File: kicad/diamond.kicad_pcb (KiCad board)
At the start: 2 copper layers, 76.5 x 66.3 mm, 40 parts, among them J1 INPUT, Q1 BD139, Q2 BD140, Q3 NJW0281G, Q4 NJW0302G, U1 NE5532

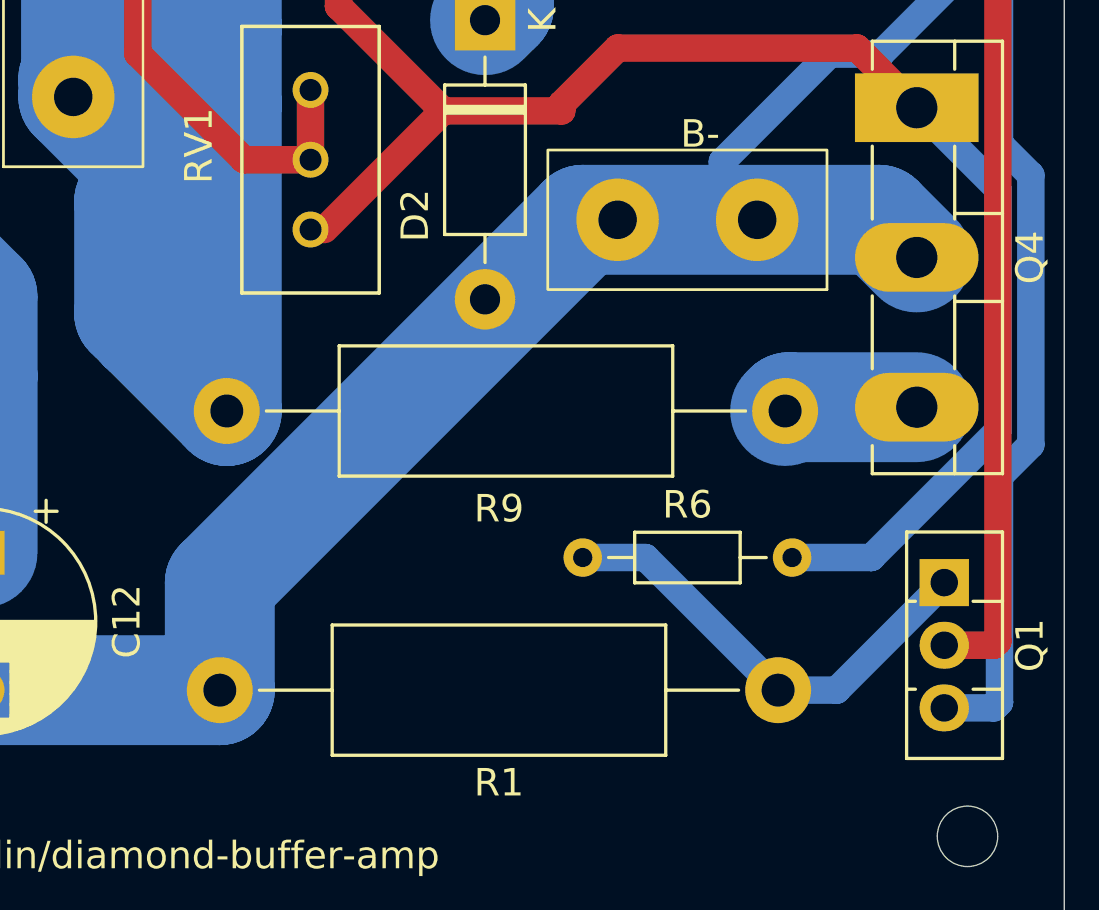
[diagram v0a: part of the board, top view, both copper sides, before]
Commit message: WIP
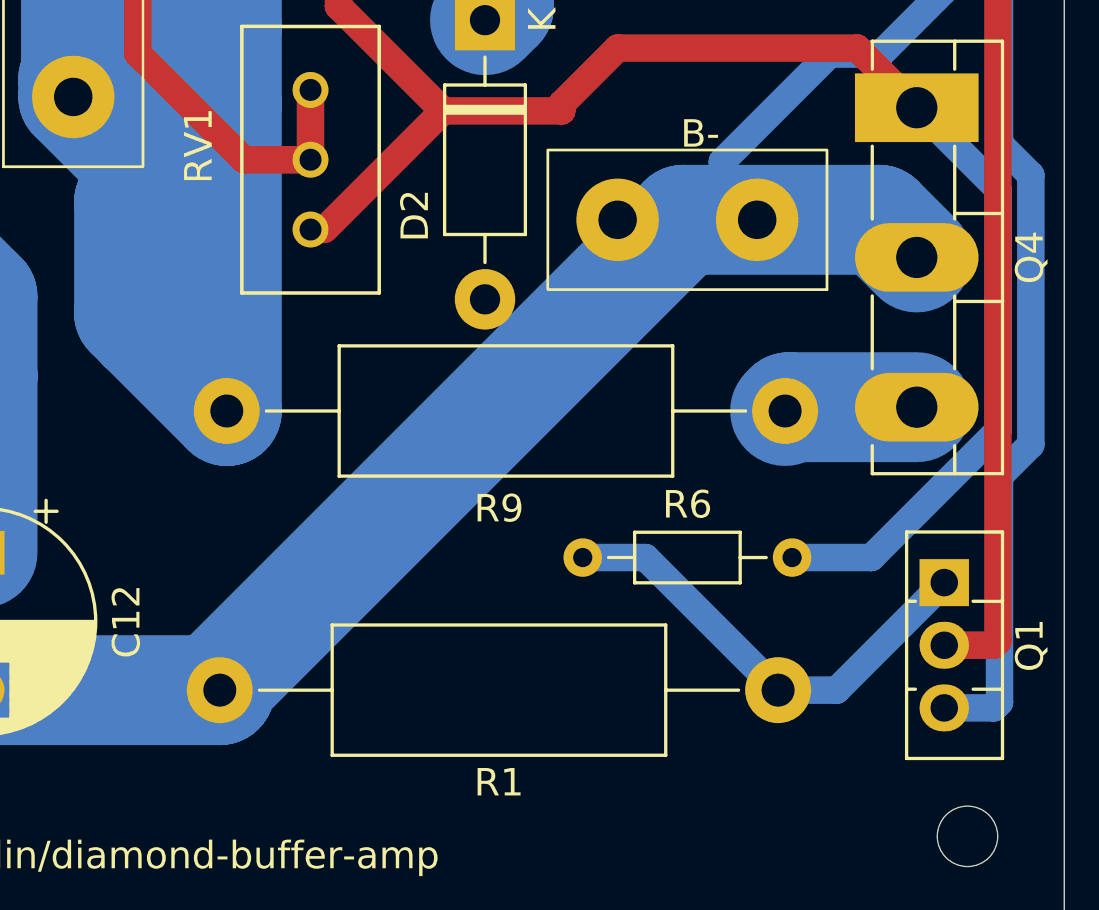
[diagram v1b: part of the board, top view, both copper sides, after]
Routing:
- net B-: track 126.9 -> 124.7 mm
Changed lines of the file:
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@@
 			(outputformat 1)
 			(mirror no)
-			(drillshape 1)
+			(drillshape 0)
 			(scaleselection 1)
-			(outputdirectory "")
+			(outputdirectory "gerber")
 		)
 	)
@@
 	)
 	(segment
-		(start 145.288 102.77)
-		(end 158.496 89.562)
-		(width 4)
+		(start 171.654 58.298)
+		(end 170.053 59.899)
+		(width 1)
 		(layer "B.Cu")
 		(net 18)
 	)
 	(segment
-		(start 171.654 58.298)
-		(end 170.053 59.899)
-		(width 1)
+		(start 145.288 106.68)
+		(end 145.288 106.426)
+		(width 4)
 		(layer "B.Cu")
 		(net 18)
@@
 	)
 	(segment
+		(start 145.288 106.426)
+		(end 162.152 89.562)
+		(width 4)
+		(layer "B.Cu")
+		(net 18)
+	)
+	(segment
+		(start 169.284 89.562)
+		(end 170.654 90.932)
+		(width 4)
+		(layer "B.Cu")
+		(net 18)
+	)
+	(segment
 		(start 169.337791 83.531)
 		(end 167.48568 83.531)
@@
 	)
 	(segment
-		(start 145.288 106.68)
-		(end 145.288 102.77)
+		(start 162.152 89.562)
+		(end 169.284 89.562)
 		(width 4)
 		(layer "B.Cu")
@@
 	)
 	(segment
-		(start 169.284 89.562)
-		(end 170.654 90.932)
-		(width 4)
-		(layer "B.Cu")
-		(net 18)
-	)
-	(segment
 		(start 170.053 59.899)
 		(end 170.053 61.575)
@@
 		(layer "B.Cu")
 		(net 18)
-	)
-	(segment
-		(start 158.496 89.562)
-		(end 169.284 89.562)
-		(width 4)
-		(layer "B.Cu")
-		(net 18)

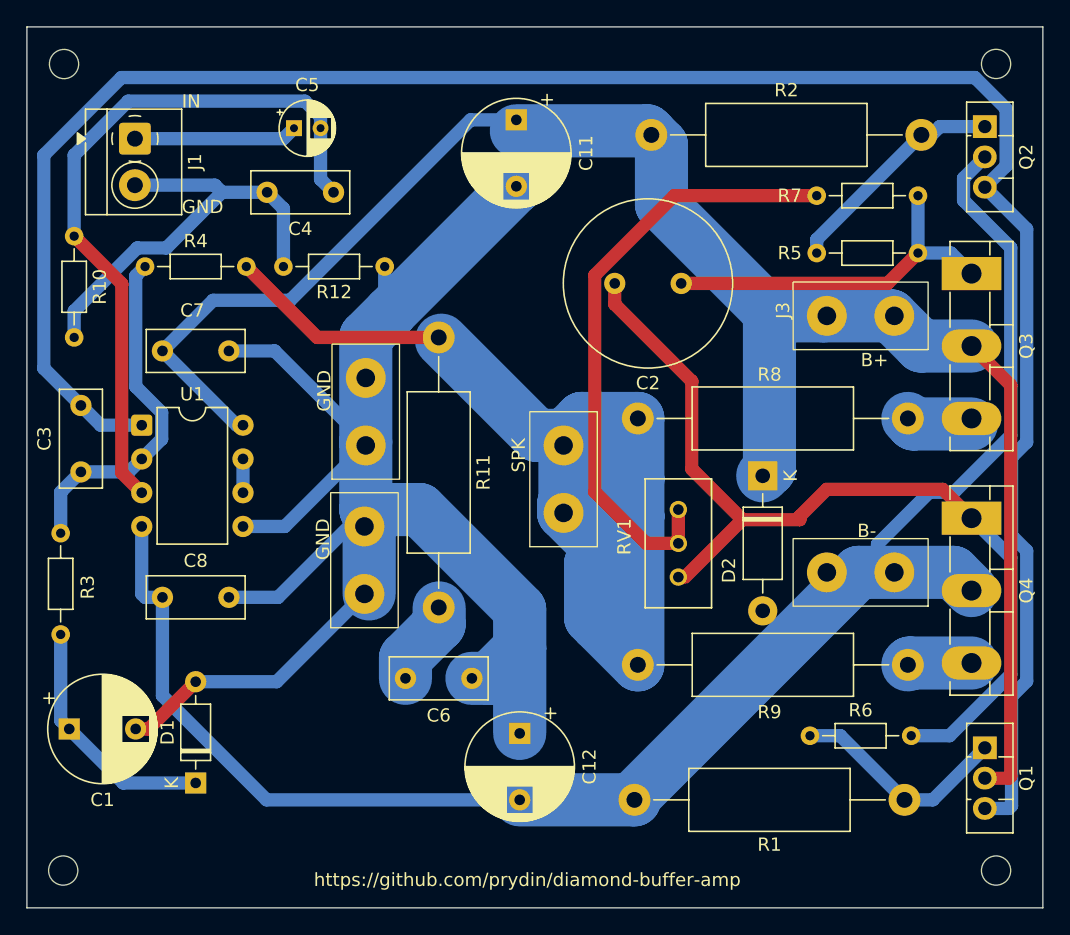
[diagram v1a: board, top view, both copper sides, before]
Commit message: WIP
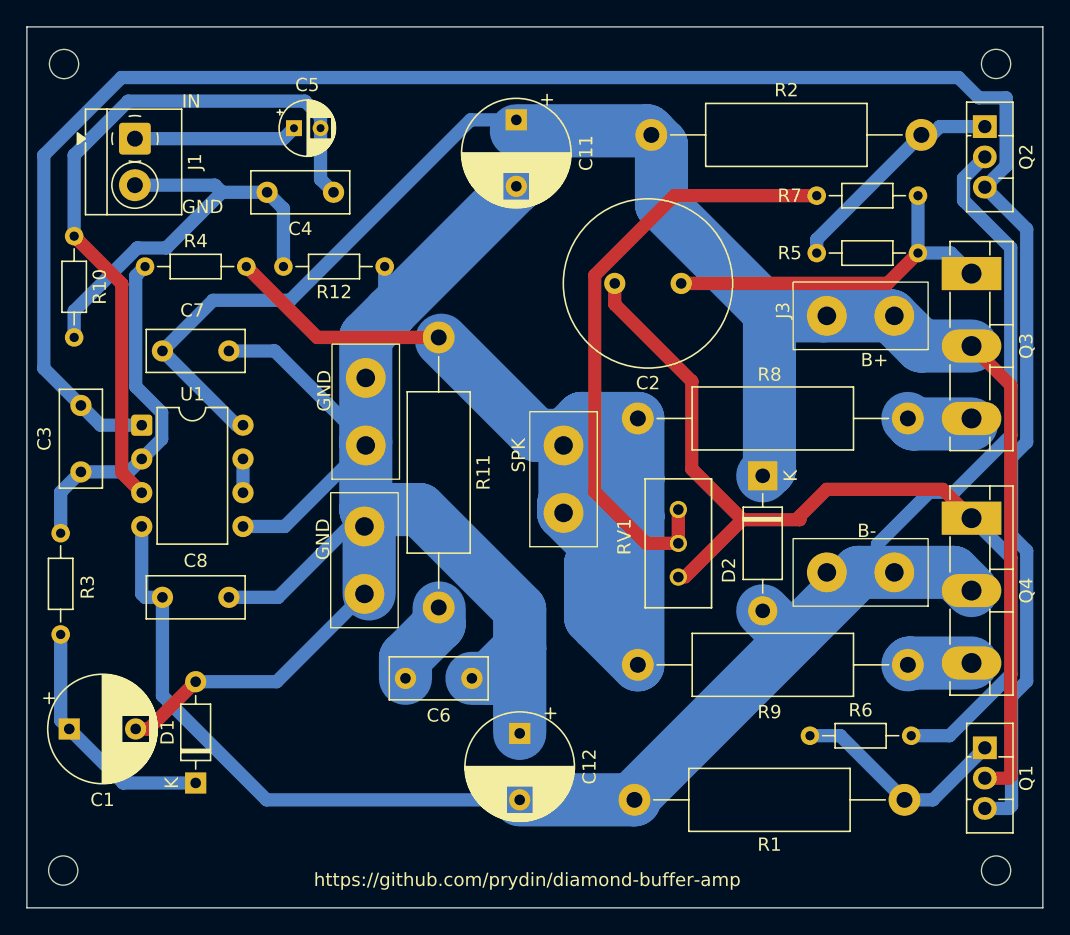
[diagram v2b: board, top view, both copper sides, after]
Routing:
- net B-: track 124.7 -> 128.0 mm
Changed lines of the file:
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@@
 	)
 	(segment
-		(start 173.255 54.672709)
-		(end 173.255 58.977)
+		(start 169.672 52.324)
+		(end 171.196 53.848)
+		(width 1)
+		(layer "B.Cu")
+		(net 3)
+	)
+	(segment
+		(start 100.838 58.166)
+		(end 106.68 52.324)
+		(width 1)
+		(layer "B.Cu")
+		(net 3)
+	)
+	(segment
+		(start 106.68 52.324)
+		(end 169.672 52.324)
 		(width 1)
 		(layer "B.Cu")
@@
 	)
 	(segment
+		(start 173.255 53.848)
+		(end 173.255 58.977)
+		(width 1)
+		(layer "B.Cu")
+		(net 3)
+	)
+	(segment
+		(start 171.196 53.848)
+		(end 173.255 53.848)
+		(width 1)
+		(layer "B.Cu")
+		(net 3)
+	)
+	(segment
+		(start 174.805 79.760847)
+		(end 174.805 63.729)
+		(width 1)
+		(layer "B.Cu")
+		(net 3)
+	)
+	(segment
+		(start 171.654 107.326)
+		(end 173.464 107.326)
+		(width 1)
+		(layer "B.Cu")
+		(net 3)
+	)
+	(segment
+		(start 173.666 86.796944)
+		(end 173.666 80.899847)
+		(width 1)
+		(layer "B.Cu")
+		(net 3)
+	)
+	(segment
+		(start 108.209 78.486)
+		(end 105.116 78.486)
+		(width 1)
+		(layer "B.Cu")
+		(net 3)
+	)
+	(segment
+		(start 103.632 77.002)
+		(end 100.838 74.208)
+		(width 1)
+		(layer "B.Cu")
+		(net 3)
+	)
+	(segment
+		(start 105.116 78.486)
+		(end 103.632 77.002)
+		(width 1)
+		(layer "B.Cu")
+		(net 3)
+	)
+	(segment
+		(start 174.805 97.747847)
+		(end 174.805 87.935944)
+		(width 1)
+		(layer "B.Cu")
+		(net 3)
+	)
+	(segment
 		(start 173.255 58.977)
 		(end 171.654 60.578)
@@
 	)
 	(segment
-		(start 174.805 79.760847)
-		(end 174.805 63.729)
-		(width 1)
-		(layer "B.Cu")
-		(net 3)
-	)
-	(segment
-		(start 171.654 107.326)
-		(end 173.464 107.326)
-		(width 1)
-		(layer "B.Cu")
-		(net 3)
-	)
-	(segment
-		(start 173.666 86.796944)
-		(end 173.666 80.899847)
-		(width 1)
-		(layer "B.Cu")
-		(net 3)
-	)
-	(segment
-		(start 108.209 78.486)
-		(end 105.116 78.486)
-		(width 1)
-		(layer "B.Cu")
-		(net 3)
-	)
-	(segment
-		(start 105.116 78.486)
-		(end 103.632 77.002)
-		(width 1)
-		(layer "B.Cu")
-		(net 3)
-	)
-	(segment
 		(start 100.838 74.208)
 		(end 100.838 58.166)
@@
 	)
 	(segment
-		(start 174.805 97.747847)
-		(end 174.805 87.935944)
-		(width 1)
-		(layer "B.Cu")
-		(net 3)
-	)
-	(segment
-		(start 103.632 77.002)
-		(end 100.838 74.208)
-		(width 1)
-		(layer "B.Cu")
-		(net 3)
-	)
-	(segment
-		(start 106.68 52.324)
-		(end 170.906291 52.324)
-		(width 1)
-		(layer "B.Cu")
-		(net 3)
-	)
-	(segment
-		(start 100.838 58.166)
-		(end 106.68 52.324)
-		(width 1)
-		(layer "B.Cu")
-		(net 3)
-	)
-	(segment
 		(start 173.464 107.326)
 		(end 173.666 107.124)
@@
 	)
 	(segment
-		(start 170.906291 52.324)
-		(end 173.255 54.672709)
-		(width 1)
-		(layer "B.Cu")
-		(net 3)
-	)
-	(segment
 		(start 174.805 87.935944)
 		(end 173.666 86.796944)
@@
 	)
 	(segment
+		(start 157.48 94.234)
+		(end 162.152 89.562)
+		(width 4)
+		(layer "B.Cu")
+		(net 18)
+	)
+	(segment
 		(start 109.768 91.44)
 		(end 109.768 98.846)
@@
 	(segment
 		(start 145.288 106.426)
-		(end 162.152 89.562)
+		(end 157.48 94.234)
 		(width 4)
 		(layer "B.Cu")
@@
 	)
 	(segment
+		(start 157.48 94.234)
+		(end 156.718 94.234)
+		(width 4)
+		(layer "B.Cu")
+		(net 18)
+	)
+	(segment
 		(start 173.605 79.263791)
 		(end 169.337791 83.531)
@@
 		(layer "B.Cu")
 		(net 18)
+	)
+	(segment
+		(start 156.718 94.234)
+		(end 154.94 92.456)
+		(width 4)
+		(layer "B.Cu")
+		(net 18)
